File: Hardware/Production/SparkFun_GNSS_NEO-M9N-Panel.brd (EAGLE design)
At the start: 135.2 x 149.5 mm, 468 parts, among them J1 MICROMOD_STANDARD, J10 MICROMOD_STANDARD, J12 Bus Selection, J14 MICROMOD_STANDARD, J16 Bus Selection, J18 MICROMOD_STANDARD, J20 Bus Selection, J22 MICROMOD_STANDARD, J24 Bus Selection, J4 Bus Selection, J6 MICROMOD_STANDARD, J8 Bus Selection, U1 U-BLOX_NEO-M9N, U10 U-BLOX_NEO-M9N, U11 EEPROM, U12 74HC1G04, U13 3.3V, U14 U-BLOX_NEO-M9N, U15 EEPROM, U16 74HC1G04, U17 3.3V, U18 U-BLOX_NEO-M9N, U19 EEPROM, U2 3.3V, U20 74HC1G04, U21 3.3V, U22 U-BLOX_NEO-M9N, U23 EEPROM, U24 74HC1G04, U3 EEPROM, U4 74HC1G04, U5 3.3V, U6 U-BLOX_NEO-M9N, U7 EEPROM, U8 74HC1G04, U9 3.3V

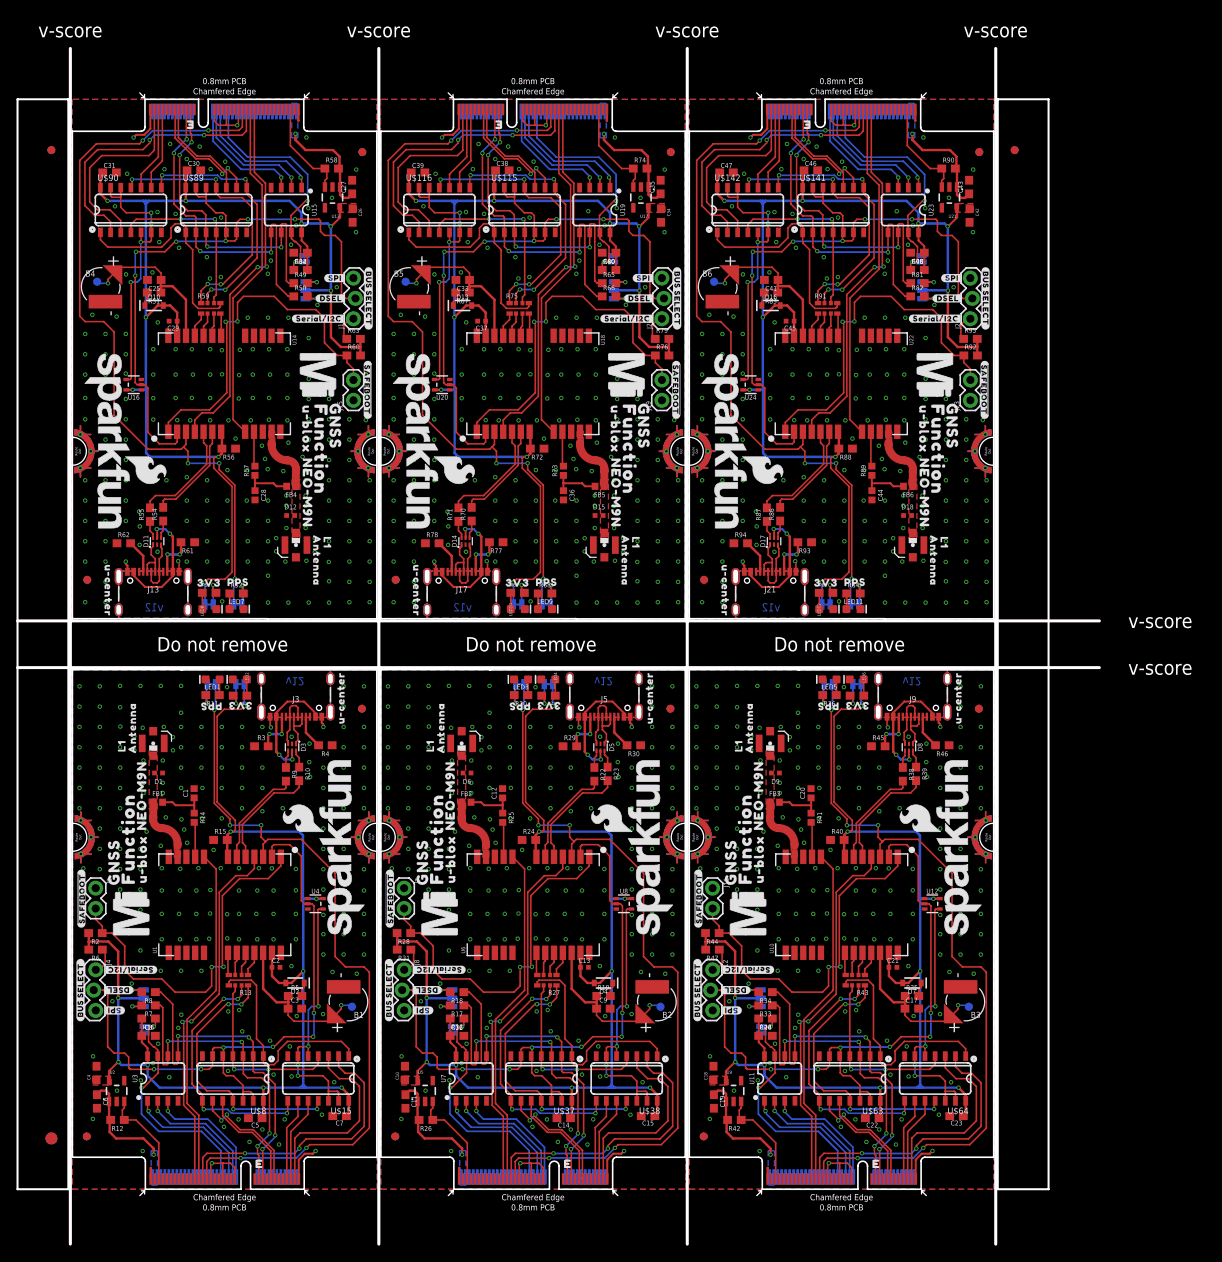
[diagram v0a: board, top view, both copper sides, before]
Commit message: Revised panel
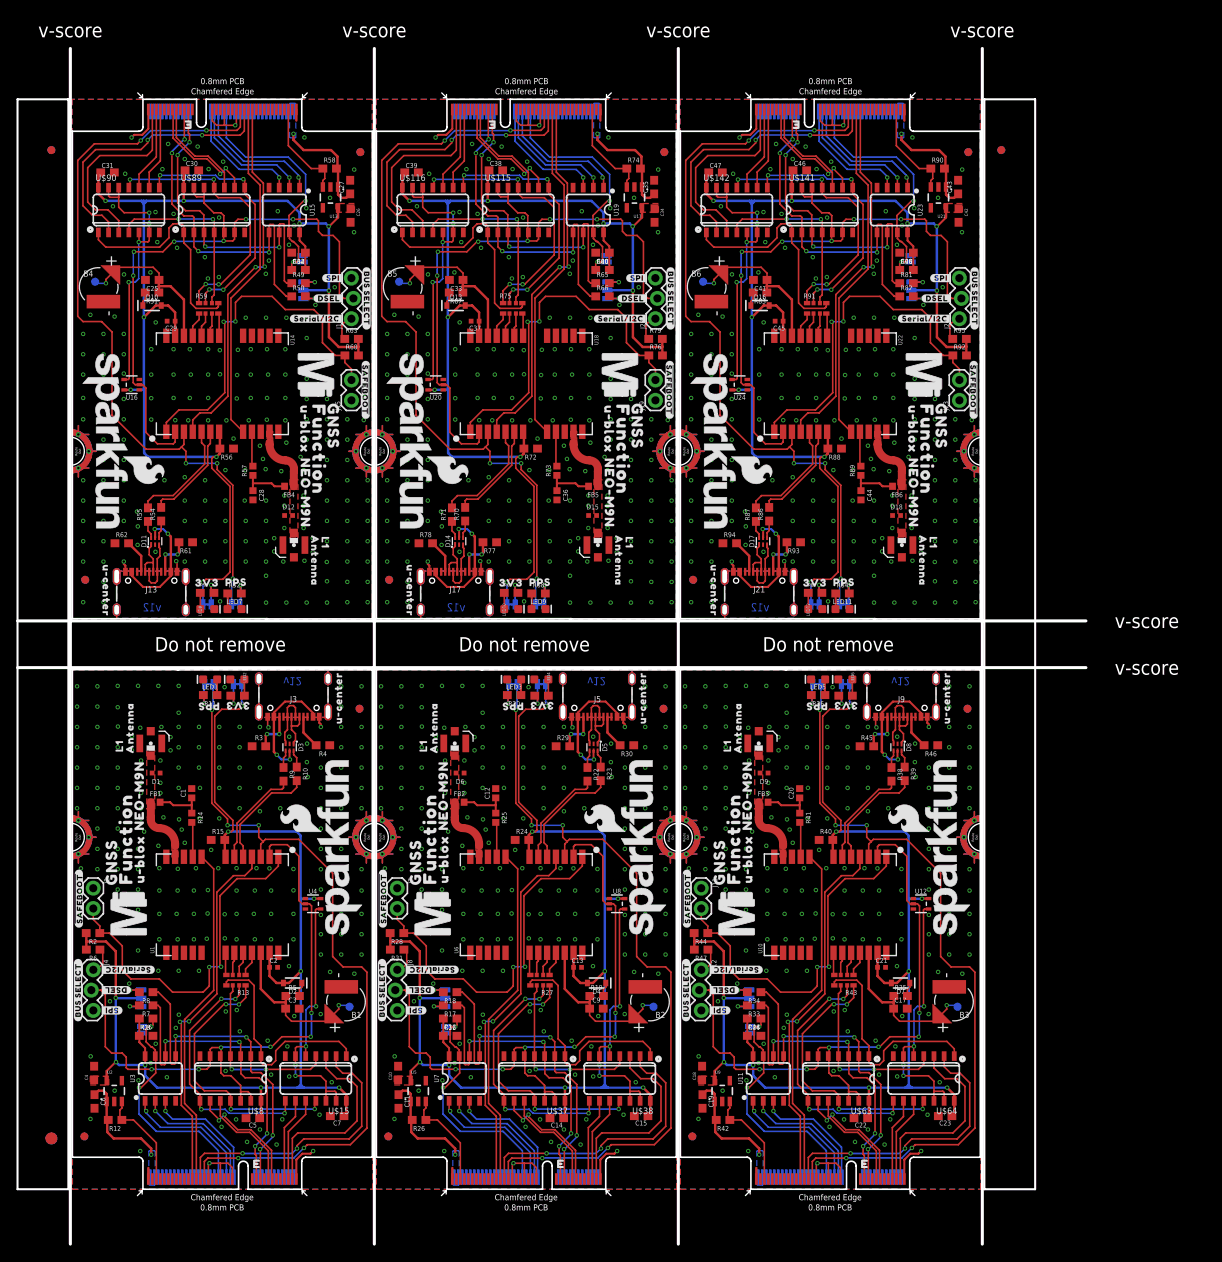
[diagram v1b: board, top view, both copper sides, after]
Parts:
- J1, J10, J14, J18, J22, J6: value MICROMOD_STANDARD -> MICROMOD_FUNCTION_STANDARD; device SparkFun-MicroMod-Function:M.2-CARD-E-22_FUNCTION_STANDARD -> SparkFun-MicroMod:M.2-CARD-E-22_FUNCTION_STANDARD
- U1, U10, U14, U18, U22, U6: device SparkFun-GPS:NEO-M9N/M8T/M8U -> SparkFun-GPS:NEO-M9N/M8T/M8U/D9S
- moved E$3 1.68 mm to (116.1, 129.9)
- moved E$4 1.68 mm to (116.1, 129.9)
- moved C21 1.42 mm to (101.1, 27.7)
- moved D7 1.42 mm to (103.5, 25.8)
- moved FB3 1.42 mm to (86.4, 48.4)
- moved LOGO6 1.42 mm to (111.3, 10.2)
- moved R35 1.42 mm to (103.5, 24.2)
- moved R39 1.42 mm to (104.0, 51.9)
- moved R42 1.42 mm to (81.3, 8.66)
- moved R43 1.42 mm to (96.4, 26.2)
- moved R44 1.42 mm to (78.6, 32.0)
- moved R45 1.42 mm to (99.3, 55.4)
- moved TP3 1.42 mm to (110.6, 22.8)
- moved U$54 1.42 mm to (93.0, 60.4)
- moved U$55 1.42 mm to (84.4, 41.2)
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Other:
- board size 135.2 x 149.5 mm -> 133.6 x 149.5 mm
